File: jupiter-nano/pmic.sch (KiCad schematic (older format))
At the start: 51 parts, among them Q1 BSS138, Q2 BSS138, Q3 BSS138, Q4 BSS138, Q5 BSS138, U2 ACT8945AQJ305-T

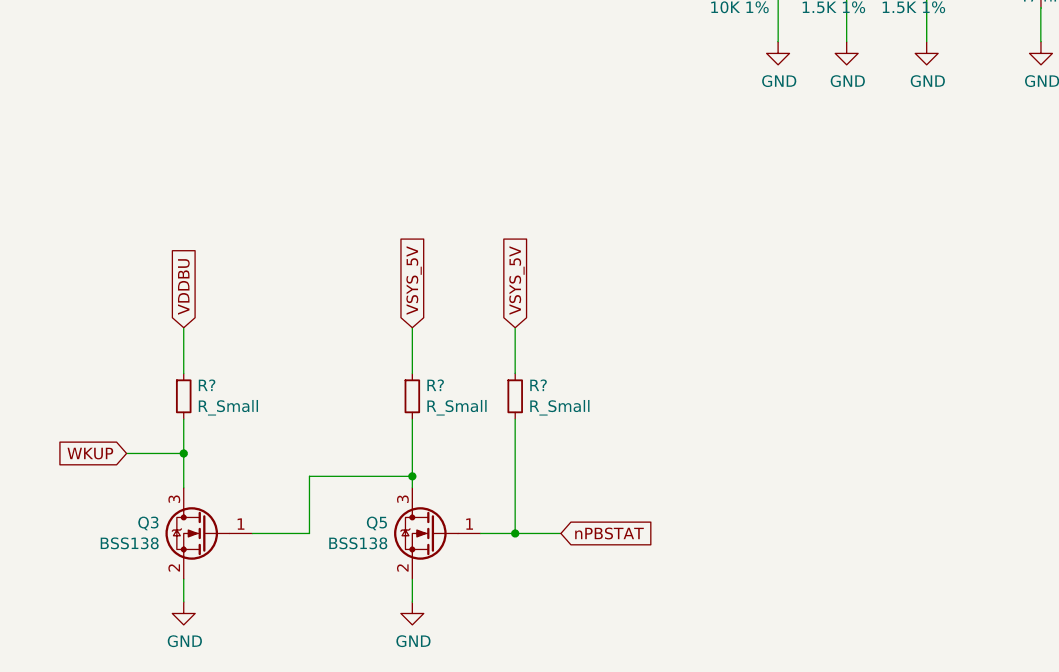
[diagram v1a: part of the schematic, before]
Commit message: WIP clocking done
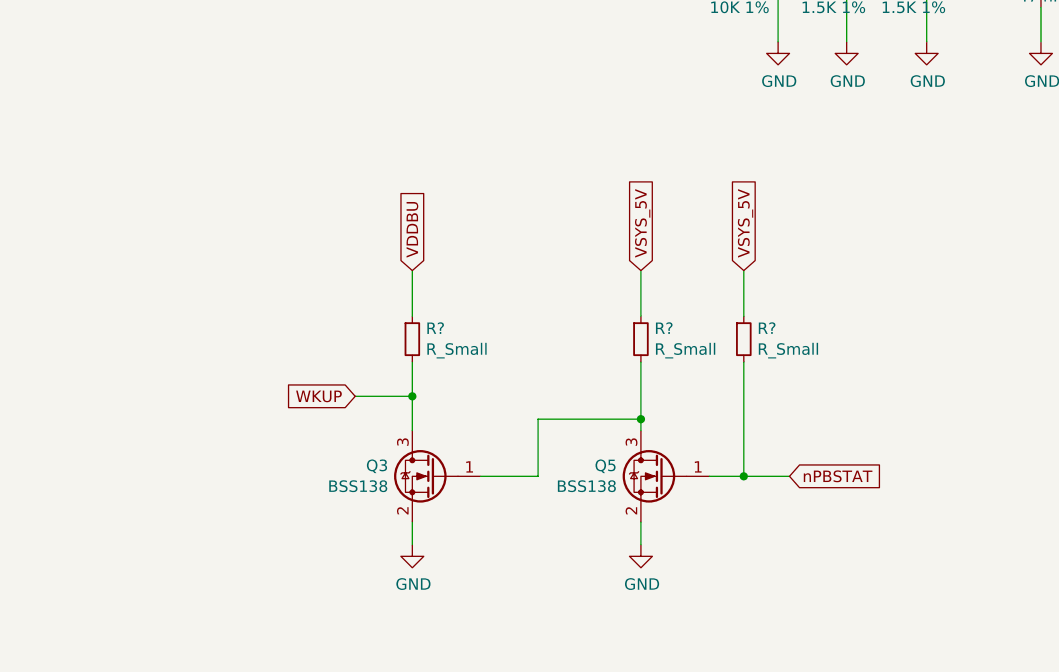
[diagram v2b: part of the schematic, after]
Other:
- moved on the sheet: Q3, Q5, R?
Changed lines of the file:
@@
 L Transistor_FET:BSS138 Q3
 U 1 1 5F66BE91
-P 1300 7150
-F 0 "Q3" H 1505 7196 50  0000 L CNN
-F 1 "BSS138" H 1505 7105 50  0000 L CNN
-F 2 "Package_TO_SOT_SMD:SOT-23" H 1500 7075 50  0001 L CIN
-F 3 "https://www.fairchildsemi.com/datasheets/BS/BSS138.pdf" H 1300 7150 50  0001 L CNN
-	1    1300 7150
+P 2300 6900
+F 0 "Q3" H 2505 6946 50  0000 L CNN
+F 1 "BSS138" H 2505 6855 50  0000 L CNN
+F 2 "Package_TO_SOT_SMD:SOT-23" H 2500 6825 50  0001 L CIN
+F 3 "https://www.fairchildsemi.com/datasheets/BS/BSS138.pdf" H 2300 6900 50  0001 L CNN
+	1    2300 6900
 	-1   0    0    -1
 $EndComp
@@
 L Transistor_FET:BSS138 Q5
 U 1 1 5F684C12
-P 2300 7150
-F 0 "Q5" H 2505 7196 50  0000 L CNN
-F 1 "BSS138" H 2505 7105 50  0000 L CNN
-F 2 "Package_TO_SOT_SMD:SOT-23" H 2500 7075 50  0001 L CIN
-F 3 "https://www.fairchildsemi.com/datasheets/BS/BSS138.pdf" H 2300 7150 50  0001 L CNN
-	1    2300 7150
+P 3300 6900
+F 0 "Q5" H 3505 6946 50  0000 L CNN
+F 1 "BSS138" H 3505 6855 50  0000 L CNN
+F 2 "Package_TO_SOT_SMD:SOT-23" H 3500 6825 50  0001 L CIN
+F 3 "https://www.fairchildsemi.com/datasheets/BS/BSS138.pdf" H 3300 6900 50  0001 L CNN
+	1    3300 6900
 	-1   0    0    -1
 $EndComp
 Wire Wire Line
-	2200 6950 2200 6900
+	3200 6700 3200 6650
 Wire Wire Line
-	2200 6900 1750 6900
+	3200 6650 2750 6650
 Wire Wire Line
-	1750 6900 1750 7150
+	2750 6650 2750 6900
 Wire Wire Line
-	1750 7150 1500 7150
+	2750 6900 2500 6900
 Wire Wire Line
-	2200 7350 2200 7450
+	3200 7100 3200 7200
 Wire Wire Line
-	1200 7350 1200 7450
+	2200 7100 2200 7200
 $Comp
 L power:GND #PWR?
 U 1 1 5F6CBF6E
-P 1200 7450
-F 0 "#PWR?" H 1200 7200 50  0001 C CNN
-F 1 "GND" H 1205 7277 50  0000 C CNN
-F 2 "" H 1200 7450 50  0001 C CNN
-F 3 "" H 1200 7450 50  0001 C CNN
-	1    1200 7450
+P 2200 7200
+F 0 "#PWR?" H 2200 6950 50  0001 C CNN
+F 1 "GND" H 2205 7027 50  0000 C CNN
+F 2 "" H 2200 7200 50  0001 C CNN
+F 3 "" H 2200 7200 50  0001 C CNN
+	1    2200 7200
 	1    0    0    -1
 $EndComp
@@
 L power:GND #PWR?
 U 1 1 5F6CCAD6
-P 2200 7450
-F 0 "#PWR?" H 2200 7200 50  0001 C CNN
-F 1 "GND" H 2205 7277 50  0000 C CNN
-F 2 "" H 2200 7450 50  0001 C CNN
-F 3 "" H 2200 7450 50  0001 C CNN
-	1    2200 7450
+P 3200 7200
+F 0 "#PWR?" H 3200 6950 50  0001 C CNN
+F 1 "GND" H 3205 7027 50  0000 C CNN
+F 2 "" H 3200 7200 50  0001 C CNN
+F 3 "" H 3200 7200 50  0001 C CNN
+	1    3200 7200
 	1    0    0    -1
 $EndComp
 Wire Wire Line
-	2500 7150 2650 7150
-Text GLabel 2850 7150 2    50   Input ~ 0
+	3500 6900 3650 6900
+Text GLabel 3850 6900 2    50   Input ~ 0
 nPBSTAT
 Wire Wire Line
-	2200 6900 2200 6650
-Connection ~ 2200 6900
+	3200 6650 3200 6400
+Connection ~ 3200 6650
 Wire Wire Line
-	2650 7150 2650 6650
-Connection ~ 2650 7150
+	3650 6900 3650 6400
+Connection ~ 3650 6900
 Wire Wire Line
-	2650 7150 2850 7150
+	3650 6900 3850 6900
 Wire Wire Line
-	1200 6950 1200 6800
-Text GLabel 2650 6250 1    50   Input ~ 0
+	2200 6700 2200 6550
+Text GLabel 3650 6000 1    50   Input ~ 0
 VSYS_5V
-Text GLabel 2200 6250 1    50   Input ~ 0
+Text GLabel 3200 6000 1    50   Input ~ 0
 VSYS_5V
-Text GLabel 1200 6250 1    50   Input ~ 0
+Text GLabel 2200 6000 1    50   Input ~ 0
 VDDBU
 $Comp
 L Device:R_Small R?
 U 1 1 5F7027C3
-P 2650 6550
-F 0 "R?" H 2709 6596 50  0000 L CNN
-F 1 "R_Small" H 2709 6505 50  0000 L CNN
-F 2 "" H 2650 6550 50  0001 C CNN
-F 3 "~" H 2650 6550 50  0001 C CNN
-	1    2650 6550
+P 3650 6300
+F 0 "R?" H 3709 6346 50  0000 L CNN
+F 1 "R_Small" H 3709 6255 50  0000 L CNN
+F 2 "" H 3650 6300 50  0001 C CNN
+F 3 "~" H 3650 6300 50  0001 C CNN
+	1    3650 6300
 	1    0    0    -1
 $EndComp
@@
 L Device:R_Small R?
 U 1 1 5F70325F
-P 2200 6550
-F 0 "R?" H 2259 6596 50  0000 L CNN
-F 1 "R_Small" H 2259 6505 50  0000 L CNN
-F 2 "" H 2200 6550 50  0001 C CNN
-F 3 "~" H 2200 6550 50  0001 C CNN
-	1    2200 6550
+P 3200 6300
+F 0 "R?" H 3259 6346 50  0000 L CNN
+F 1 "R_Small" H 3259 6255 50  0000 L CNN
+F 2 "" H 3200 6300 50  0001 C CNN
+F 3 "~" H 3200 6300 50  0001 C CNN
+	1    3200 6300
 	1    0    0    -1
 $EndComp
@@
 L Device:R_Small R?
 U 1 1 5F703D5F
-P 1200 6550
-F 0 "R?" H 1259 6596 50  0000 L CNN
-F 1 "R_Small" H 1259 6505 50  0000 L CNN
-F 2 "" H 1200 6550 50  0001 C CNN
-F 3 "~" H 1200 6550 50  0001 C CNN
-	1    1200 6550
+P 2200 6300
+F 0 "R?" H 2259 6346 50  0000 L CNN
+F 1 "R_Small" H 2259 6255 50  0000 L CNN
+F 2 "" H 2200 6300 50  0001 C CNN
+F 3 "~" H 2200 6300 50  0001 C CNN
+	1    2200 6300
 	1    0    0    -1
 $EndComp
-Connection ~ 1200 6800
+Connection ~ 2200 6550
 Wire Wire Line
-	1200 6800 1200 6650
+	2200 6550 2200 6400
 Wire Wire Line
-	1200 6250 1200 6450
+	2200 6000 2200 6200
 Wire Wire Line
-	2200 6250 2200 6450
+	3200 6000 3200 6200
 Wire Wire Line
-	2650 6250 2650 6450
+	3650 6000 3650 6200
 Wire Wire Line
-	950  6800 1200 6800
-Text GLabel 950  6800 0    50   Input ~ 0
+	1950 6550 2200 6550
+Text GLabel 1950 6550 0    50   Input ~ 0
 WKUP
 $Comp
